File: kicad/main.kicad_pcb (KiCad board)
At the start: 2 copper layers, 97.8 x 97.8 mm, 48 parts, among them J1 Jack-DC, J2 LCD, J3 Bus, J4 PWR, J5 uSD, J6 VIA_B, J7 IO~{EN}_{[2..7]}, J8 Control, P1 Mini-DIN-6, SW1 Step, SW2 Reset, U1 74HC00, U2 74HC00, X1 4 MHz

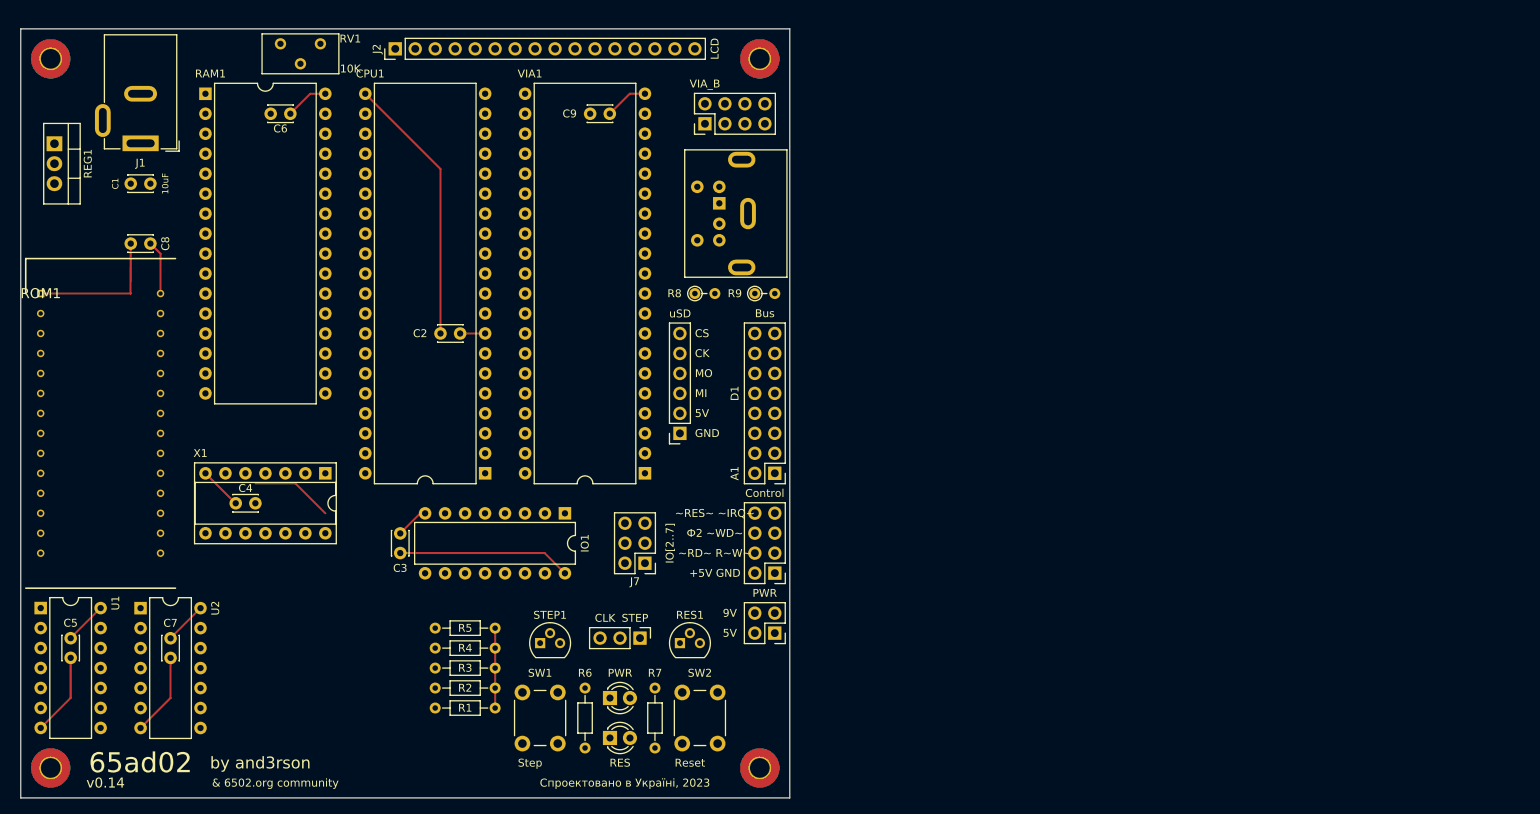
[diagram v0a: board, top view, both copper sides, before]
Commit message: WIP: v0.15
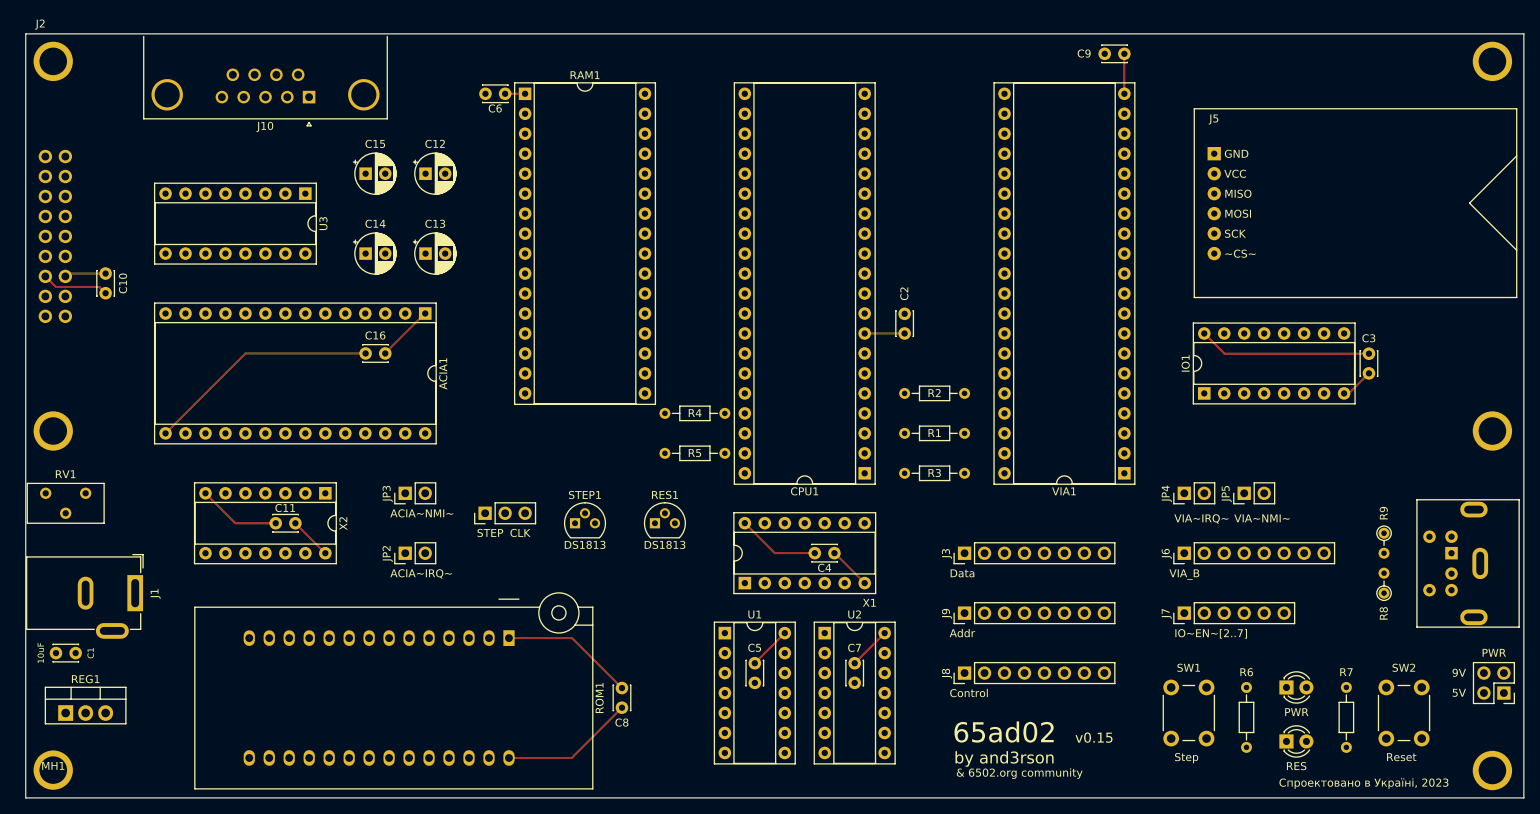
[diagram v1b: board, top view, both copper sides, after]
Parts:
- removed REF** (x4): MountingHole_2.5mm_Pad_TopBottom, MountingHole:MountingHole_2.5mm_Pad_TopBottom
- added ACIA1: W65C51N6TPG, Package_DIP:DIP-28_W15.24mm_Socket, F.Cu at (71.1, 53.3)
- added C10: 0.1uF, Capacitor_THT:C_Disc_D3.0mm_W2.0mm_P2.50mm, F.Cu at (30.5, 48.3)
- added C11: 0,1uF, Capacitor_THT:C_Disc_D3.0mm_W2.0mm_P2.50mm, F.Cu at (52.1, 80.0)
- added C12: 10uF, Capacitor_THT:CP_Radial_D5.0mm_P2.50mm, F.Cu at (71.2, 35.6)
- added C13: 10uF, Capacitor_THT:CP_Radial_D5.0mm_P2.50mm, F.Cu at (71.2, 45.7)
- added C14: 10uF, Capacitor_THT:CP_Radial_D5.0mm_P2.50mm, F.Cu at (63.5, 45.7)
- added C15: 10uF, Capacitor_THT:CP_Radial_D5.0mm_P2.50mm, F.Cu at (63.5, 35.6)
- added C16: 0.1uF, Capacitor_THT:C_Disc_D3.0mm_W2.0mm_P2.50mm, F.Cu at (63.5, 58.4)
- added J10: RS232, Connector_Dsub:DSUB-9_Male_Horizontal_P2.77x2.84mm_EdgePinOffset4.94mm_Housed_MountingHolesOffset7.48mm, F.Cu at (56.4, 25.8)
- added J9: Addr, Connector_PinHeader_2.54mm:PinHeader_1x08_P2.54mm_Vertical, F.Cu at (139.7, 91.4)
- added JP2: ACIA~{IRQ}, Connector_PinHeader_2.54mm:PinHeader_1x02_P2.54mm_Vertical, F.Cu at (68.6, 83.8)
- added JP3: ACIA~{NMI}, Connector_PinHeader_2.54mm:PinHeader_1x02_P2.54mm_Vertical, F.Cu at (68.6, 76.2)
- added JP4: VIA~{IRQ}, Connector_PinHeader_2.54mm:PinHeader_1x02_P2.54mm_Vertical, F.Cu at (167.6, 76.2)
- added JP5: VIA~{NMI}, Connector_PinHeader_2.54mm:PinHeader_1x02_P2.54mm_Vertical, F.Cu at (175.3, 76.2)
- added MH1: MountingHole, my:Hole_3.5x5, F.Cu at (23.8, 111.4)
- added MH2: MountingHole, my:Hole_3.5x5, F.Cu at (206.8, 111.5)
- added U3: MAX232, Package_DIP:DIP-16_W7.62mm_Socket, F.Cu at (55.9, 38.1)
- added X2: 1.8432 MHz, Package_DIP:DIP-14_W7.62mm_Socket, F.Cu at (58.4, 76.2)
- CPU1, VIA1: footprint Package_DIP:DIP-40_W15.24mm -> Package_DIP:DIP-40_W15.24mm_Socket
- IO1: footprint Package_DIP:DIP-16_W7.62mm -> Package_DIP:DIP-16_W7.62mm_Socket
- J2: value LCD -> LCD_Conn; footprint Connector_PinHeader_2.54mm:PinHeader_1x16_P2.54mm_Vertical -> my:LCD_4004
- J3: value Bus -> Data; footprint Connector_PinHeader_2.54mm:PinHeader_2x08_P2.54mm_Vertical -> Connector_PinHeader_2.54mm:PinHeader_1x08_P2.54mm_Vertical
- J5: footprint Connector_PinSocket_2.54mm:PinSocket_1x06_P2.54mm_Vertical -> my:MicroSD-Adapter
- J6, J8: footprint Connector_PinHeader_2.54mm:PinHeader_2x04_P2.54mm_Vertical -> Connector_PinHeader_2.54mm:PinHeader_1x08_P2.54mm_Vertical
- J7: footprint Connector_PinHeader_2.54mm:PinHeader_2x03_P2.54mm_Vertical -> Connector_PinHeader_2.54mm:PinHeader_1x06_P2.54mm_Vertical
- RAM1: footprint Package_DIP:DIP-32_W15.24mm -> Package_DIP:DIP-32_W15.24mm_Socket
- ROM1: footprint 28-526-10:DIPS1524W61P254L4191H673Q28N -> Socket:DIP_Socket-28_W11.9_W12.7_W15.24_W17.78_W18.5_3M_228-1277-00-0602J
- U1, U2: footprint Package_DIP:DIP-14_W7.62mm -> Package_DIP:DIP-14_W7.62mm_Socket
- moved C3 124.8 mm to (191.1, 61.0), turned to 90 degrees
- moved P1 103.2 mm to (201.6, 83.8)
- moved R8 95.6 mm to (193.0, 88.9), turned to 90 degrees
- moved J4 93.0 mm to (208.3, 101.6)
- moved SW2 89.5 mm to (193.3, 107.4)
- moved R7 87.9 mm to (188.2, 100.9)
- moved C5 87.1 mm to (113.0, 97.8)
- moved U1 87.1 mm to (109.2, 94.0)
- moved C7 87.1 mm to (125.7, 97.8)
- moved U2 87.1 mm to (121.9, 94.0)
- moved D1 86.0 mm to (180.6, 100.9)
- moved D2 86.0 mm to (180.6, 107.8)
- moved R9 85.6 mm to (193.0, 81.3), turned to -90 degrees
- moved C8 84.2 mm to (96.1, 101.0), turned to -90 degrees
- moved R6 84.1 mm to (175.6, 108.5)
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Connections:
- net Net-(CPU1-~{NMI}) renamed ~{NMI}
- IO1 pad 14: unconnected-(IO1-O1-Pad14) -> ACIA~{EN}
- J2 pad 1: GND -> unconnected-(J2-Pin_1-Pad1)
- J2 pad 10: unconnected-(J2-Pin_10-Pad10) -> LCDR~{W}
- J2 pad 11: PA_{0} -> LCDRS
- J2 pad 12: PA_{1} -> Net-(J2-Pin_12)
- J2 pad 13: PA_{2} -> GND
- J2 pad 14: PA_{3} -> +5V
- J2 pad 15: +5V -> LCDEN2
- J2 pad 16: GND -> unconnected-(J2-Pin_16-Pad16)
- J2 pad 2: +5V -> unconnected-(J2-Pin_2-Pad2)
- J2 pad 3: Net-(J2-Pin_3) -> unconnected-(J2-Pin_3-Pad3)
- J2 pad 4: PA_{6} -> unconnected-(J2-Pin_4-Pad4)
- J2 pad 5: PA_{5} -> LCDD4
- J2 pad 6: PA_{4} -> LCDD5
- J2 pad 7: unconnected-(J2-Pin_7-Pad7) -> LCDD6
- J2 pad 8: unconnected-(J2-Pin_8-Pad8) -> LCDD7
- J2 pad 9: unconnected-(J2-Pin_9-Pad9) -> LCDEN1
- J3 pad 1: A_{0} -> D_{0}
- J3 pad 2: A_{1} -> D_{1}
- J3 pad 3: A_{2} -> D_{2}
- J3 pad 4: A_{3} -> D_{3}
- J3 pad 5: A_{4} -> D_{4}
- J3 pad 6: A_{5} -> D_{5}
- J3 pad 7: A_{6} -> D_{6}
- J3 pad 8: A_{7} -> D_{7}
- J6 pad 7: Net-(J6-Pin_7) -> +5V
- J6 pad 8: Net-(J6-Pin_8) -> GND
- P1 pad 1: PA_{7} -> PS2DATA
- P1 pad 5: CA1 -> PS2CLK
- R8 pad 1: CA1 -> PS2CLK
- R9 pad 1: PA_{7} -> PS2DATA
- RV1 pad 2: Net-(J2-Pin_3) -> Net-(J2-Pin_12)
- VIA1 pad 14: Net-(J6-Pin_3) -> PS2DATA
- VIA1 pad 15: Net-(J6-Pin_4) -> Net-(J6-Pin_3)
- VIA1 pad 16: Net-(J6-Pin_5) -> Net-(J6-Pin_4)
- VIA1 pad 17: Net-(J6-Pin_6) -> Net-(J6-Pin_5)
- VIA1 pad 18: Net-(J6-Pin_7) -> PS2CLK
- VIA1 pad 19: Net-(J6-Pin_8) -> Net-(J6-Pin_6)
- VIA1 pad 2: PA_{0} -> LCDD4
- VIA1 pad 21: ~{IRQ} -> Net-(JP4-B)
- VIA1 pad 3: PA_{1} -> LCDD5
- VIA1 pad 4: PA_{2} -> LCDD6
- VIA1 pad 40: CA1 -> unconnected-(VIA1-CA1-Pad40)
- VIA1 pad 5: PA_{3} -> LCDD7
- VIA1 pad 6: PA_{4} -> LCDEN1
- VIA1 pad 7: PA_{5} -> LCDEN2
- VIA1 pad 8: PA_{6} -> LCDR~{W}
- VIA1 pad 9: PA_{7} -> LCDRS
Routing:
- net +5V: track 74.5 -> 113.3 mm
- net GND: track 82.8 -> 52.9 mm
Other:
- board size 97.8 x 97.8 mm -> 190.5 x 97.2 mm
- board text added: "ACIA~IRQ~"
- board text added: "ACIA~NMI~"
- board text added: "Addr"
- board text added: "Control"
- board text added: "Data"
- board text added: "IO~EN~[2..7]"
- board text added: "VIA_B"
- board text added: "VIA~IRQ~"
- board text added: "VIA~NMI~"
- board text added: "v0.15"
- board text removed: "v0.14"
